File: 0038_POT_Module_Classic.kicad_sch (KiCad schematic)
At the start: 12 parts

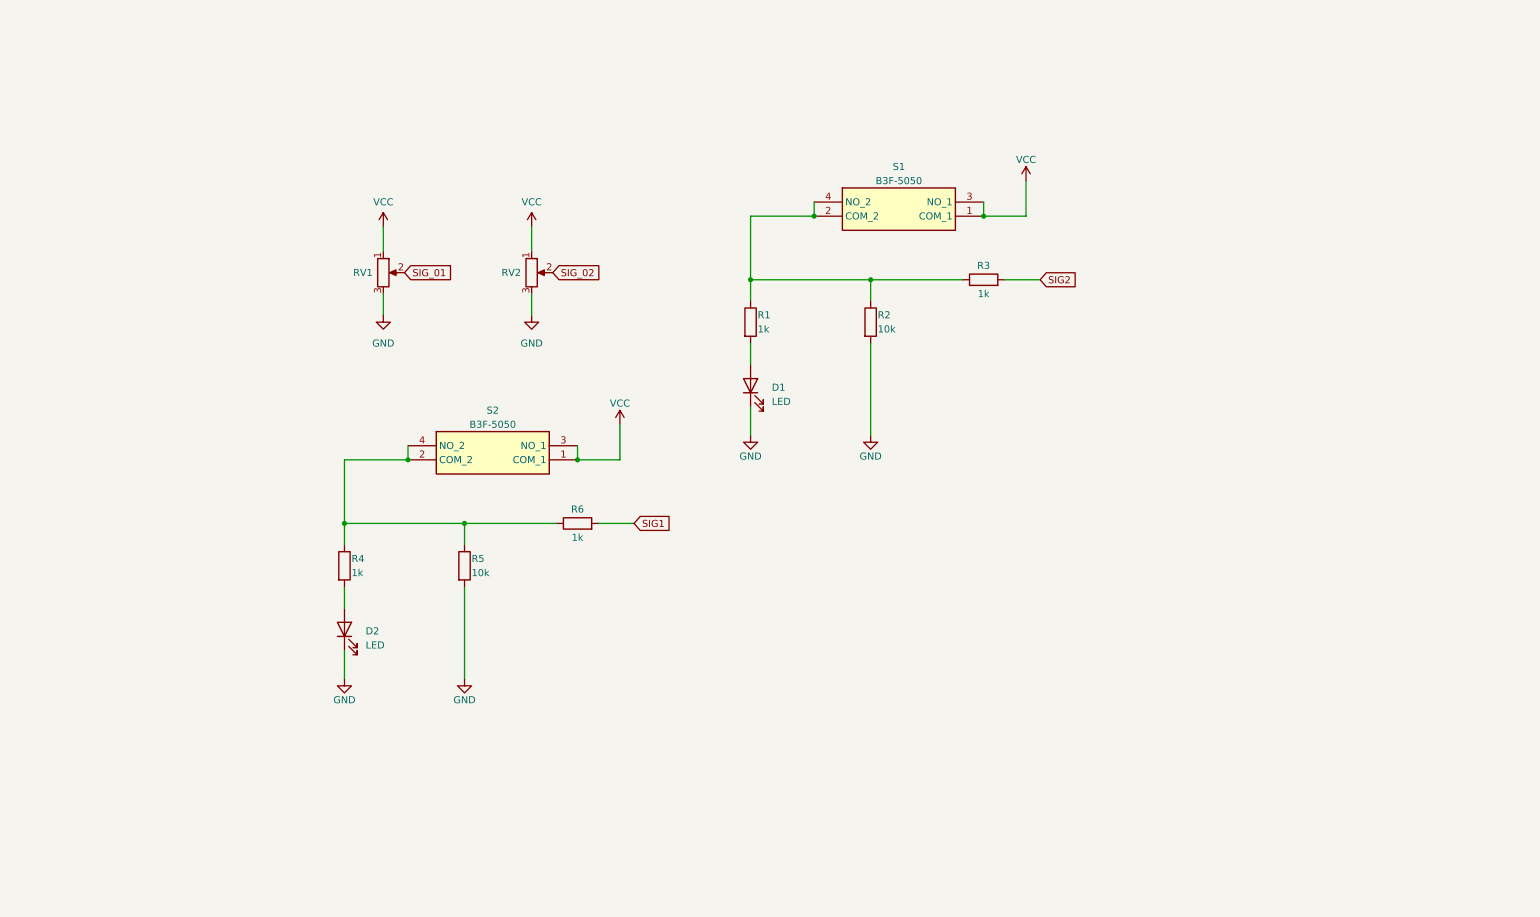
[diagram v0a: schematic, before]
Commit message: Add files via upload
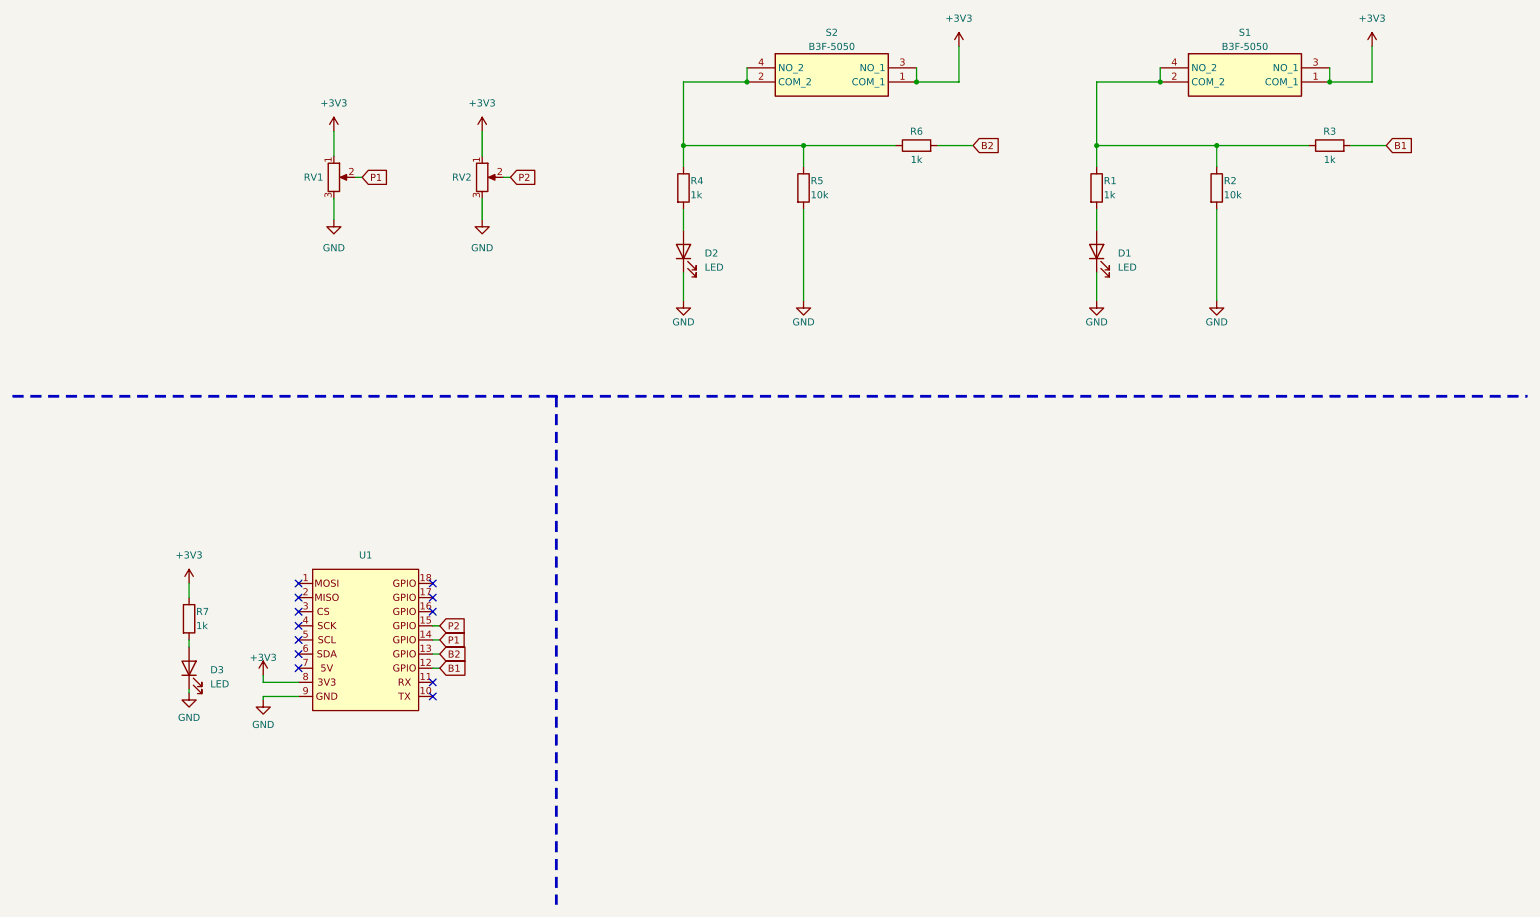
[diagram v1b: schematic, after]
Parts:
- added D3: LED, LED_SMD:LED_0603_1608Metric, symbol Device:LED
- added R7: 1k, Resistor_SMD:R_0603_1608Metric, symbol Device:R
- added U1: ~, Moduler_:pin_header_5-3, symbol moduler_pin:air
- D1, D2: footprint (none) -> LED_SMD:LED_0603_1608Metric
- R1, R2, R3, R4, R5, R6: footprint (none) -> Resistor_SMD:R_0603_1608Metric
- RV1, RV2: footprint (none) -> meminle:RK09D113F25C0B504
- S1, S2: footprint B3F-4055 -> meminle:B3F-4055
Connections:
- net GND: now also D3.1 (K), U1.9
- net SIG1 renamed B2
- net B2: now also U1.13
- net SIG2 renamed B1
- net B1: now also U1.12
- net SIG_01 renamed P1
- net P1: now also U1.14
- net SIG_02 renamed P2
- net P2: now also U1.15
- net VCC renamed +3V3
- net +3V3: now also R7.1, U1.8
- new net: D3.2 (A), R7.2
- no-connect marks 0 -> 12
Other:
- moved on the sheet: D1, D2, R1, R2, R3, R4, R5, R6, RV1, RV2, S1, S2
